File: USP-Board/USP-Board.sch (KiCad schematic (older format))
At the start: 6 parts

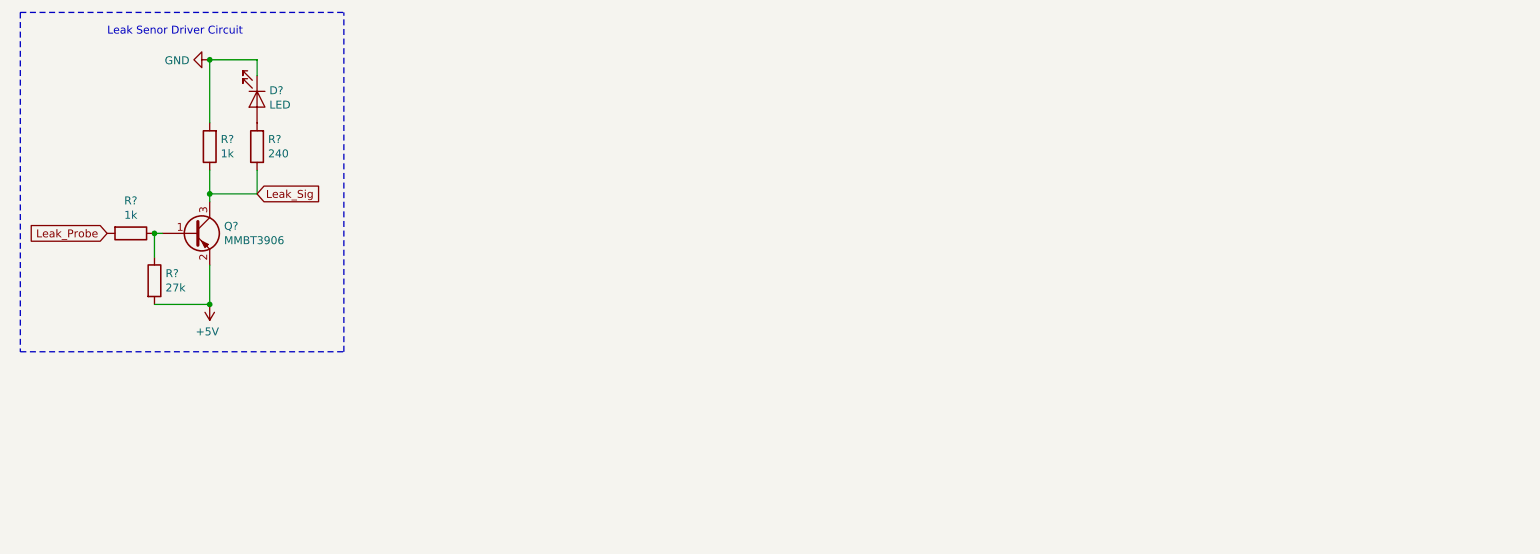
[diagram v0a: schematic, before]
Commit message: Worked on USp Sch needs more work
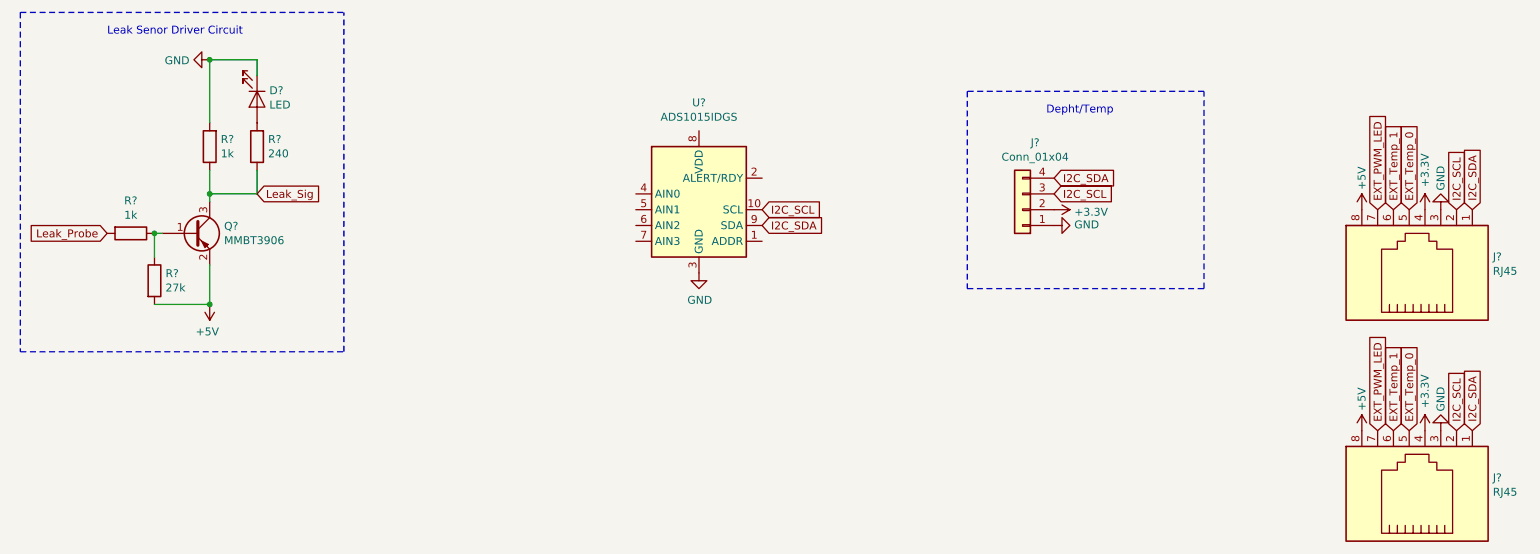
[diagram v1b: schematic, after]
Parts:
- added J? (x2): RJ45, symbol Connector:RJ45
- added J?: Conn_01x04, symbol Connector_Generic:Conn_01x04
- added U?: ADS1015IDGS, Package_SO:TSSOP-10_3x3mm_P0.5mm, symbol Analog_ADC:ADS1015IDGS
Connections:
- net +5V: now also J?.8, J?.8
- net GND: now also J?.1 (Pin_1), J?.3, J?.3, U?.3 (GND)
- new net +3V3: J?.2 (Pin_2), J?.4, J?.4
- new net EXT_PWM_LED: J?.7, J?.7
- new net EXT_Temp_0: J?.5, J?.5
- new net EXT_Temp_1: J?.6, J?.6
- new net I2C_SCL: J?.2, J?.2, J?.3 (Pin_3), U?.10 (SCL)
- new net I2C_SDA: J?.1, J?.1, J?.4 (Pin_4), U?.9 (SDA)
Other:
- note added: "Depht/Temp\n"
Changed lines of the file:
@@
 Wire Notes Line
 	950  700  3000 700
+$Comp
+L Connector:RJ45 J?
+U 1 1 5C6DE016
+P 9850 2350
+F 0 "J?" V 9952 1920 50  0000 R CNN
+F 1 "RJ45" V 9861 1920 50  0000 R CNN
+F 2 "" V 9850 2375 50  0001 C CNN
+F 3 "~" V 9850 2375 50  0001 C CNN
+	1    9850 2350
+	0    -1   -1   0
+$EndComp
+$Comp
+L power:+5V #PWR?
+U 1 1 5C6DE0A6
+P 9450 1950
+F 0 "#PWR?" H 9450 1800 50  0001 C CNN
+F 1 "+5V" V 9450 2150 50  0000 C CNN
+F 2 "" H 9450 1950 50  0001 C CNN
+F 3 "" H 9450 1950 50  0001 C CNN
+	1    9450 1950
+	1    0    0    -1
+$EndComp
+Text GLabel 9550 1950 1    50   Input ~ 0
+EXT_PWM_LED
+Text GLabel 9650 1950 1    50   Input ~ 0
+EXT_Temp_1
+Text GLabel 9750 1950 1    50   Input ~ 0
+EXT_Temp_0
+$Comp
+L power:+3.3V #PWR?
+U 1 1 5C6DE2D4
+P 9850 1950
+F 0 "#PWR?" H 9850 1800 50  0001 C CNN
+F 1 "+3.3V" V 9850 2200 50  0000 C CNN
+F 2 "" H 9850 1950 50  0001 C CNN
+F 3 "" H 9850 1950 50  0001 C CNN
+	1    9850 1950
+	1    0    0    -1
+$EndComp
+$Comp
+L power:GND #PWR?
+U 1 1 5C6DE388
+P 9950 1950
+F 0 "#PWR?" H 9950 1700 50  0001 C CNN
+F 1 "GND" V 9950 1750 50  0000 C CNN
+F 2 "" H 9950 1950 50  0001 C CNN
+F 3 "" H 9950 1950 50  0001 C CNN
+	1    9950 1950
+	-1   0    0    1
+$EndComp
+Text GLabel 10050 1950 1    50   Input ~ 0
+I2C_SCL
+Text GLabel 10150 1950 1    50   Input ~ 0
+I2C_SDA
+$Comp
+L Connector:RJ45 J?
+U 1 1 5C6DE972
+P 9850 3750
+F 0 "J?" V 9952 3320 50  0000 R CNN
+F 1 "RJ45" V 9861 3320 50  0000 R CNN
+F 2 "" V 9850 3775 50  0001 C CNN
+F 3 "~" V 9850 3775 50  0001 C CNN
+	1    9850 3750
+	0    -1   -1   0
+$EndComp
+$Comp
+L power:+5V #PWR?
+U 1 1 5C6DE979
+P 9450 3350
+F 0 "#PWR?" H 9450 3200 50  0001 C CNN
+F 1 "+5V" V 9450 3550 50  0000 C CNN
+F 2 "" H 9450 3350 50  0001 C CNN
+F 3 "" H 9450 3350 50  0001 C CNN
+	1    9450 3350
+	1    0    0    -1
+$EndComp
+Text GLabel 9550 3350 1    50   Input ~ 0
+EXT_PWM_LED
+Text GLabel 9650 3350 1    50   Input ~ 0
+EXT_Temp_1
+Text GLabel 9750 3350 1    50   Input ~ 0
+EXT_Temp_0
+$Comp
+L power:+3.3V #PWR?
+U 1 1 5C6DE982
+P 9850 3350
+F 0 "#PWR?" H 9850 3200 50  0001 C CNN
+F 1 "+3.3V" V 9850 3600 50  0000 C CNN
+F 2 "" H 9850 3350 50  0001 C CNN
+F 3 "" H 9850 3350 50  0001 C CNN
+	1    9850 3350
+	1    0    0    -1
+$EndComp
+$Comp
+L power:GND #PWR?
+U 1 1 5C6DE988
+P 9950 3350
+F 0 "#PWR?" H 9950 3100 50  0001 C CNN
+F 1 "GND" V 9950 3150 50  0000 C CNN
+F 2 "" H 9950 3350 50  0001 C CNN
+F 3 "" H 9950 3350 50  0001 C CNN
+	1    9950 3350
+	-1   0    0    1
+$EndComp
+Text GLabel 10050 3350 1    50   Input ~ 0
+I2C_SCL
+Text GLabel 10150 3350 1    50   Input ~ 0
+I2C_SDA
+$Comp
+L Analog_ADC:ADS1015IDGS U?
+U 1 1 5C6DF5CB
+P 5250 1950
+F 0 "U?" H 5250 2628 50  0000 C CNN
+F 1 "ADS1015IDGS" H 5250 2537 50  0000 C CNN
+F 2 "Package_SO:TSSOP-10_3x3mm_P0.5mm" H 5250 1450 50  0001 C CNN
+F 3 "http://www.ti.com/lit/ds/symlink/ads1015.pdf" H 5200 1050 50  0001 C CNN
+	1    5250 1950
+	1    0    0    -1
+$EndComp
+Text GLabel 5650 1950 2    50   Input ~ 0
+I2C_SCL
+Text GLabel 5650 2050 2    50   Input ~ 0
+I2C_SDA
+$Comp
+L power:GND #PWR?
+U 1 1 5C6E015F
+P 5250 2350
+F 0 "#PWR?" H 5250 2100 50  0001 C CNN
+F 1 "GND" H 5255 2177 50  0000 C CNN
+F 2 "" H 5250 2350 50  0001 C CNN
+F 3 "" H 5250 2350 50  0001 C CNN
+	1    5250 2350
+	1    0    0    -1
+$EndComp
+$Comp
+L Connector_Generic:Conn_01x04 J?
+U 1 1 5C6E0A3E
+P 7300 1950
+F 0 "J?" H 7220 1525 50  0000 C CNN
+F 1 "Conn_01x04" H 7220 1616 50  0000 C CNN
+F 2 "" H 7300 1950 50  0001 C CNN
+F 3 "~" H 7300 1950 50  0001 C CNN
+	1    7300 1950
+	-1   0    0    1
+$EndComp
+$Comp
+L power:GND #PWR?
+U 1 1 5C6E0F3C
+P 7500 2050
+F 0 "#PWR?" H 7500 1800 50  0001 C CNN
+F 1 "GND" V 7505 1922 50  0000 R CNN
+F 2 "" H 7500 2050 50  0001 C CNN
+F 3 "" H 7500 2050 50  0001 C CNN
+	1    7500 2050
+	0    -1   -1   0
+$EndComp
+$Comp
+L power:+3.3V #PWR?
+U 1 1 5C6E0F9E
+P 7500 1950
+F 0 "#PWR?" H 7500 1800 50  0001 C CNN
+F 1 "+3.3V" V 7515 2078 50  0000 L CNN
+F 2 "" H 7500 1950 50  0001 C CNN
+F 3 "" H 7500 1950 50  0001 C CNN
+	1    7500 1950
+	0    1    1    0
+$EndComp
+Text GLabel 7500 1850 2    50   Input ~ 0
+I2C_SCL
+Text GLabel 7500 1750 2    50   Input ~ 0
+I2C_SDA
+Wire Notes Line
+	6950 2450 8450 2450
+Wire Notes Line
+	8450 2450 8450 1200
+Wire Notes Line
+	8450 1200 6950 1200
+Wire Notes Line
+	6950 1200 6950 2450
+Text Notes 7450 1350 0    50   ~ 0
+Depht/Temp\n
 $EndSCHEMATC
